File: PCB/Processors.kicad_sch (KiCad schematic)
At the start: 2 parts, among them U5 STM32H753VITx

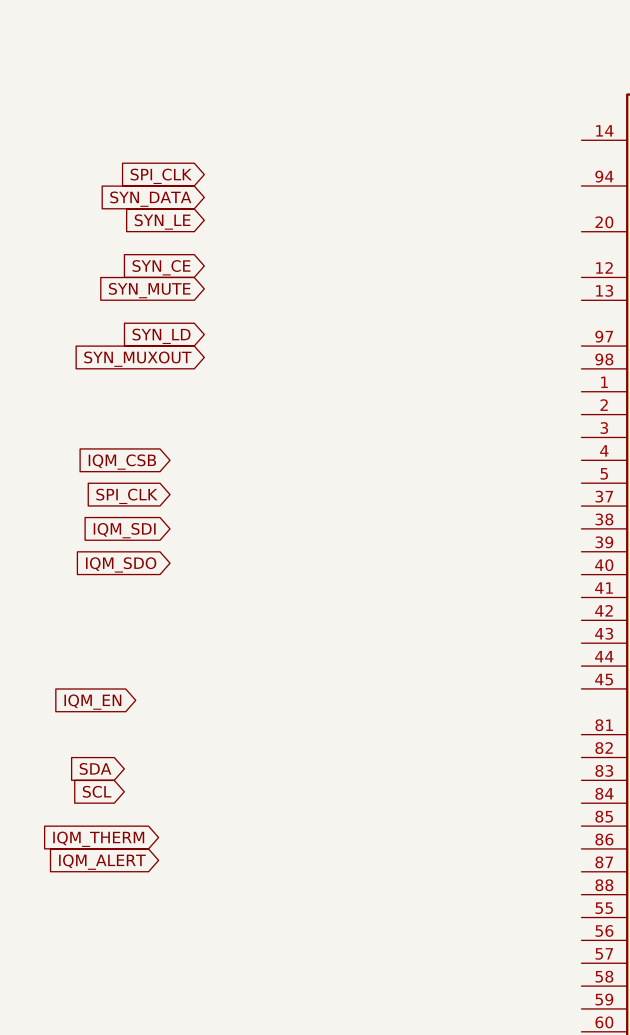
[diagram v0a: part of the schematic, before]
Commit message: Updated PCB schematics, added new datasheet and components library
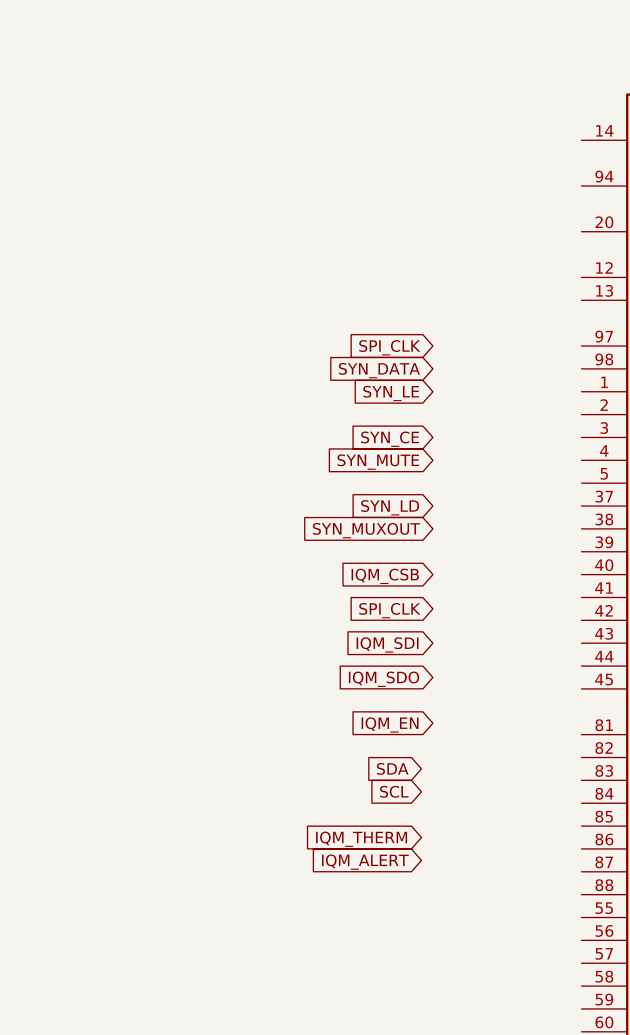
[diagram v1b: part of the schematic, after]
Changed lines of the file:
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@@
 	(global_label "SYN_LD"
 		(shape input)
-		(at 66.04 67.31 180)
-		(fields_autoplaced yes)
-		(effects
-			(font
-				(size 1.27 1.27)
-			)
-			(justify right)
-		)
-		(property "Intersheetrefs" "${INTERSHEET_REFS}"
-			(at 56.1605 67.31 0)
+		(at 91.44 86.36 180)
+		(fields_autoplaced yes)
+		(effects
+			(font
+				(size 1.27 1.27)
+			)
+			(justify right)
+		)
+		(property "Intersheetrefs" "${INTERSHEET_REFS}"
+			(at 81.5605 86.36 0)
 			(hide yes)
 			(show_name no)
@@
 	(global_label "SYN_CE"
 		(shape input)
-		(at 66.04 59.69 180)
-		(fields_autoplaced yes)
-		(effects
-			(font
-				(size 1.27 1.27)
-			)
-			(justify right)
-		)
-		(property "Intersheetrefs" "${INTERSHEET_REFS}"
-			(at 56.0396 59.69 0)
+		(at 91.44 78.74 180)
+		(fields_autoplaced yes)
+		(effects
+			(font
+				(size 1.27 1.27)
+			)
+			(justify right)
+		)
+		(property "Intersheetrefs" "${INTERSHEET_REFS}"
+			(at 81.4396 78.74 0)
 			(hide yes)
 			(show_name no)
@@
 	(global_label "SDA"
 		(shape input)
-		(at 57.15 115.57 180)
-		(fields_autoplaced yes)
-		(effects
-			(font
-				(size 1.27 1.27)
-			)
-			(justify right)
-		)
-		(property "Intersheetrefs" "${INTERSHEET_REFS}"
-			(at 50.5967 115.57 0)
+		(at 90.17 115.57 180)
+		(fields_autoplaced yes)
+		(effects
+			(font
+				(size 1.27 1.27)
+			)
+			(justify right)
+		)
+		(property "Intersheetrefs" "${INTERSHEET_REFS}"
+			(at 83.6167 115.57 0)
 			(hide yes)
 			(show_name no)
@@
 	(global_label "IQM_THERM"
 		(shape input)
-		(at 60.96 123.19 180)
-		(fields_autoplaced yes)
-		(effects
-			(font
-				(size 1.27 1.27)
-			)
-			(justify right)
-		)
-		(property "Intersheetrefs" "${INTERSHEET_REFS}"
-			(at 47.452 123.19 0)
+		(at 90.17 123.19 180)
+		(fields_autoplaced yes)
+		(effects
+			(font
+				(size 1.27 1.27)
+			)
+			(justify right)
+		)
+		(property "Intersheetrefs" "${INTERSHEET_REFS}"
+			(at 76.662 123.19 0)
 			(hide yes)
 			(show_name no)
@@
 	(global_label "SYN_LE"
 		(shape input)
-		(at 66.04 54.61 180)
-		(fields_autoplaced yes)
-		(effects
-			(font
-				(size 1.27 1.27)
-			)
-			(justify right)
-		)
-		(property "Intersheetrefs" "${INTERSHEET_REFS}"
-			(at 56.2815 54.61 0)
+		(at 91.44 73.66 180)
+		(fields_autoplaced yes)
+		(effects
+			(font
+				(size 1.27 1.27)
+			)
+			(justify right)
+		)
+		(property "Intersheetrefs" "${INTERSHEET_REFS}"
+			(at 81.6815 73.66 0)
 			(hide yes)
 			(show_name no)
@@
 	(global_label "SYN_DATA"
 		(shape input)
-		(at 66.04 52.07 180)
-		(fields_autoplaced yes)
-		(effects
-			(font
-				(size 1.27 1.27)
-			)
-			(justify right)
-		)
-		(property "Intersheetrefs" "${INTERSHEET_REFS}"
-			(at 54.0438 52.07 0)
+		(at 91.44 71.12 180)
+		(fields_autoplaced yes)
+		(effects
+			(font
+				(size 1.27 1.27)
+			)
+			(justify right)
+		)
+		(property "Intersheetrefs" "${INTERSHEET_REFS}"
+			(at 79.4438 71.12 0)
 			(hide yes)
 			(show_name no)
@@
 	(global_label "SPI_CLK"
 		(shape input)
-		(at 62.23 85.09 180)
-		(fields_autoplaced yes)
-		(effects
-			(font
-				(size 1.27 1.27)
-			)
-			(justify right)
-		)
-		(property "Intersheetrefs" "${INTERSHEET_REFS}"
-			(at 51.6248 85.09 0)
+		(at 91.44 97.79 180)
+		(fields_autoplaced yes)
+		(effects
+			(font
+				(size 1.27 1.27)
+			)
+			(justify right)
+		)
+		(property "Intersheetrefs" "${INTERSHEET_REFS}"
+			(at 80.8348 97.79 0)
 			(hide yes)
 			(show_name no)
@@
 	(global_label "SYN_MUTE"
 		(shape input)
-		(at 66.04 62.23 180)
-		(fields_autoplaced yes)
-		(effects
-			(font
-				(size 1.27 1.27)
-			)
-			(justify right)
-		)
-		(property "Intersheetrefs" "${INTERSHEET_REFS}"
-			(at 53.5601 62.23 0)
+		(at 91.44 81.28 180)
+		(fields_autoplaced yes)
+		(effects
+			(font
+				(size 1.27 1.27)
+			)
+			(justify right)
+		)
+		(property "Intersheetrefs" "${INTERSHEET_REFS}"
+			(at 78.9601 81.28 0)
 			(hide yes)
 			(show_name no)
@@
 	(global_label "IQM_SDI"
 		(shape input)
-		(at 62.23 88.9 180)
-		(fields_autoplaced yes)
-		(effects
-			(font
-				(size 1.27 1.27)
-			)
-			(justify right)
-		)
-		(property "Intersheetrefs" "${INTERSHEET_REFS}"
-			(at 51.8062 88.9 0)
+		(at 91.44 101.6 180)
+		(fields_autoplaced yes)
+		(effects
+			(font
+				(size 1.27 1.27)
+			)
+			(justify right)
+		)
+		(property "Intersheetrefs" "${INTERSHEET_REFS}"
+			(at 81.0162 101.6 0)
 			(hide yes)
 			(show_name no)
@@
 	(global_label "IQM_EN"
 		(shape input)
-		(at 58.42 107.95 180)
-		(fields_autoplaced yes)
-		(effects
-			(font
-				(size 1.27 1.27)
-			)
-			(justify right)
-		)
-		(property "Intersheetrefs" "${INTERSHEET_REFS}"
-			(at 48.601 107.95 0)
+		(at 91.44 110.49 180)
+		(fields_autoplaced yes)
+		(effects
+			(font
+				(size 1.27 1.27)
+			)
+			(justify right)
+		)
+		(property "Intersheetrefs" "${INTERSHEET_REFS}"
+			(at 81.621 110.49 0)
 			(hide yes)
 			(show_name no)
@@
 	(global_label "IQM_ALERT"
 		(shape input)
-		(at 60.96 125.73 180)
-		(fields_autoplaced yes)
-		(effects
-			(font
-				(size 1.27 1.27)
-			)
-			(justify right)
-		)
-		(property "Intersheetrefs" "${INTERSHEET_REFS}"
-			(at 48.1172 125.73 0)
+		(at 90.17 125.73 180)
+		(fields_autoplaced yes)
+		(effects
+			(font
+				(size 1.27 1.27)
+			)
+			(justify right)
+		)
+		(property "Intersheetrefs" "${INTERSHEET_REFS}"
+			(at 77.3272 125.73 0)
 			(hide yes)
 			(show_name no)
@@
 	(global_label "SCL"
 		(shape input)
-		(at 57.15 118.11 180)
-		(fields_autoplaced yes)
-		(effects
-			(font
-				(size 1.27 1.27)
-			)
-			(justify right)
-		)
-		(property "Intersheetrefs" "${INTERSHEET_REFS}"
-			(at 50.6572 118.11 0)
+		(at 90.17 118.11 180)
+		(fields_autoplaced yes)
+		(effects
+			(font
+				(size 1.27 1.27)
+			)
+			(justify right)
+		)
+		(property "Intersheetrefs" "${INTERSHEET_REFS}"
+			(at 83.6772 118.11 0)
 			(hide yes)
 			(show_name no)
@@
 	(global_label "SYN_MUXOUT"
 		(shape input)
-		(at 66.04 69.85 180)
-		(fields_autoplaced yes)
-		(effects
-			(font
-				(size 1.27 1.27)
-			)
-			(justify right)
-		)
-		(property "Intersheetrefs" "${INTERSHEET_REFS}"
-			(at 50.8386 69.85 0)
+		(at 91.44 88.9 180)
+		(fields_autoplaced yes)
+		(effects
+			(font
+				(size 1.27 1.27)
+			)
+			(justify right)
+		)
+		(property "Intersheetrefs" "${INTERSHEET_REFS}"
+			(at 76.2386 88.9 0)
 			(hide yes)
 			(show_name no)
@@
 	(global_label "IQM_CSB"
 		(shape input)
-		(at 62.23 81.28 180)
-		(fields_autoplaced yes)
-		(effects
-			(font
-				(size 1.27 1.27)
-			)
-			(justify right)
-		)
-		(property "Intersheetrefs" "${INTERSHEET_REFS}"
-			(at 51.141 81.28 0)
+		(at 91.44 93.98 180)
+		(fields_autoplaced yes)
+		(effects
+			(font
+				(size 1.27 1.27)
+			)
+			(justify right)
+		)
+		(property "Intersheetrefs" "${INTERSHEET_REFS}"
+			(at 80.351 93.98 0)
 			(hide yes)
 			(show_name no)
@@
 	(global_label "IQM_SDO"
 		(shape input)
-		(at 62.23 92.71 180)
-		(fields_autoplaced yes)
-		(effects
-			(font
-				(size 1.27 1.27)
-			)
-			(justify right)
-		)
-		(property "Intersheetrefs" "${INTERSHEET_REFS}"
-			(at 51.0805 92.71 0)
+		(at 91.44 105.41 180)
+		(fields_autoplaced yes)
+		(effects
+			(font
+				(size 1.27 1.27)
+			)
+			(justify right)
+		)
+		(property "Intersheetrefs" "${INTERSHEET_REFS}"
+			(at 80.2905 105.41 0)
 			(hide yes)
 			(show_name no)
@@
 	(global_label "SPI_CLK"
 		(shape input)
-		(at 66.04 49.53 180)
-		(fields_autoplaced yes)
-		(effects
-			(font
-				(size 1.27 1.27)
-			)
-			(justify right)
-		)
-		(property "Intersheetrefs" "${INTERSHEET_REFS}"
-			(at 55.4348 49.53 0)
-			(hide yes)
-			(show_name no)
+		(at 91.44 68.58 180)
+		(fields_autoplaced yes)
+		(effects
+			(font
+				(size 1.27 1.27)
+			)
+			(justify right)
+		)
+		(property "Intersheetrefs" "${INTERSHEET_REFS}"
+			(at 80.8348 68.58 0)
+			(hide yes)
+			(show_name no)
